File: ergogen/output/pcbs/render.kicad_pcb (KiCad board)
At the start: 2 copper layers, 220.4 x 89.6 mm, 63 parts

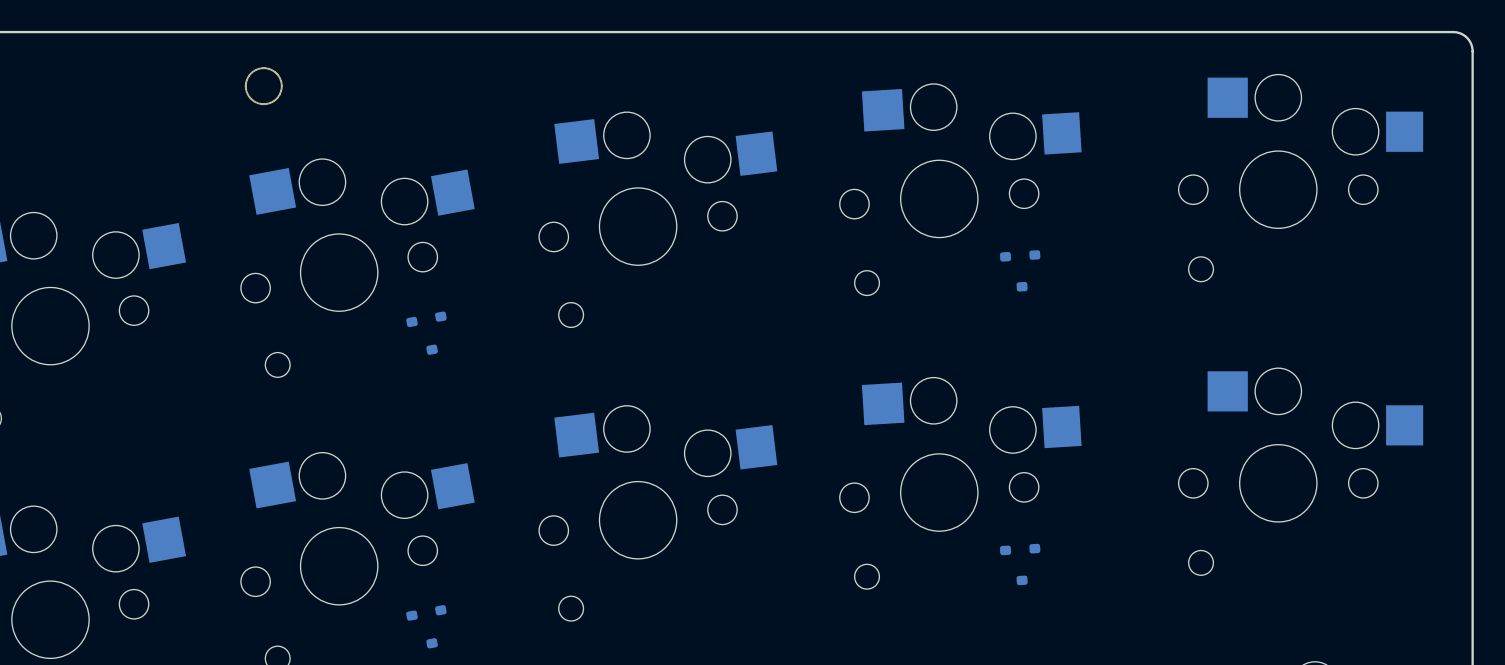
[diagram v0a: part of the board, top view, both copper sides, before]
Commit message: update
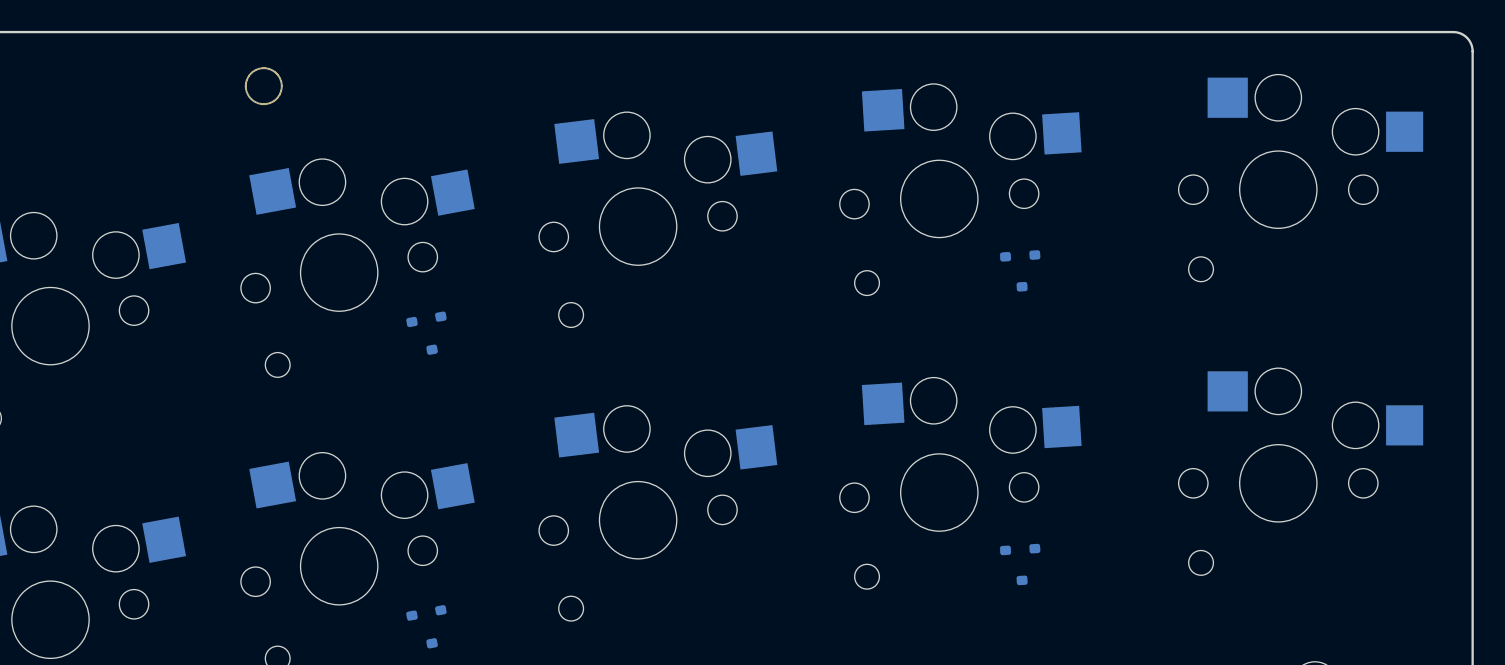
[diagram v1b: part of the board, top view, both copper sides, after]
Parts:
- XX2: footprint 1:conn_molex_pico_front -> conn_molex_pico_front
- moved SW24 141.7 mm to (197.7, 38.0), turned to 0 degrees
- moved SW19 137.6 mm to (-2.38, 38.0), turned to 0 degrees
- moved SW4 116.6 mm to (41.4, 2.39), turned to -7 degrees
- moved SW11 113.5 mm to (21.9, 19.6), turned to -3.5 degrees
- moved SW7 112.7 mm to (173.4, 0.60), turned to 3.5 degrees
- moved SW15 112.7 mm to (173.4, 19.6), turned to 3.5 degrees
- moved SW25 103.9 mm to (178.4, 38.3), turned to 1.75 degrees
- moved SW20 99.5 mm to (16.9, 38.3), turned to -1.75 degrees
- moved SW29 86.7 mm to (55.6, 65.2), turned to -10.5 degrees
- moved SW12 75.5 mm to (41.4, 21.4), turned to -7 degrees
- moved SW16 74.7 mm to (153.9, 21.4), turned to 7 degrees
- moved SW8 74.7 mm to (153.9, 2.39), turned to 7 degrees
- moved SW3 72.8 mm to (21.9, 0.60), turned to -3.5 degrees
- moved SW22 39.4 mm to (56.1, 42.5), turned to -10.5 degrees
- moved SW27 39.4 mm to (139.2, 42.5), turned to 10.5 degrees
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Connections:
- SW10 pad 1: C3 -> C5
- SW10 pad 2: mirror_e_top -> mirror_t_top
- SW11 pad 1: C4 -> C2
- SW11 pad 2: mirror_r_top -> s_home
- SW12 pad 1: C5 -> C3
- SW12 pad 2: mirror_t_top -> d_home
- SW13 pad 1: C2 -> C4
- SW13 pad 2: s_home -> f_home
- SW14 pad 1: C3 -> C5
- SW14 pad 2: d_home -> g_home
- SW15 pad 1: C4 -> C2
- SW15 pad 2: f_home -> mirror_s_home
- SW16 pad 1: C5 -> C3
- SW16 pad 2: g_home -> mirror_d_home
- SW17 pad 1: C2 -> C4
- SW17 pad 2: mirror_s_home -> mirror_f_home
- SW18 pad 1: C3 -> C5
- SW18 pad 2: mirror_d_home -> mirror_g_home
- SW19 pad 1: C4 -> C1
- SW19 pad 2: mirror_f_home -> z_bottom
- SW20 pad 1: C5 -> C2
- SW20 pad 2: mirror_g_home -> x_bottom
- SW21 pad 1: C1 -> C3
- SW21 pad 2: z_bottom -> c_bottom
- SW22 pad 1: C2 -> C4
- SW22 pad 2: x_bottom -> v_bottom
- SW23 pad 1: C3 -> C5
- SW23 pad 2: c_bottom -> b_bottom
- SW24 pad 1: C4 -> C1
- SW24 pad 2: v_bottom -> mirror_z_bottom
- SW25 pad 1: C5 -> C2
- SW25 pad 2: b_bottom -> mirror_x_bottom
- SW26 pad 1: C1 -> C3
- SW26 pad 2: mirror_z_bottom -> mirror_c_bottom
- SW27 pad 1: C2 -> C4
- SW27 pad 2: mirror_x_bottom -> mirror_v_bottom
- SW28 pad 1: C3 -> C5
- SW28 pad 2: mirror_c_bottom -> mirror_b_bottom
- SW29 pad 2: mirror_v_bottom -> base_thumb
- SW3 pad 1: C4 -> C2
- SW3 pad 2: base_thumb -> w_top
- SW30 pad 1: C5 -> C4
- SW30 pad 2: mirror_b_bottom -> mirror_base_thumb
- SW4 pad 1: C4 -> C3
- SW4 pad 2: mirror_base_thumb -> e_top
- SW5 pad 1: C2 -> C4
- SW5 pad 2: w_top -> r_top
- SW6 pad 1: C3 -> C5
- SW6 pad 2: e_top -> t_top
- SW7 pad 1: C4 -> C2
- SW7 pad 2: r_top -> mirror_w_top
- SW8 pad 1: C5 -> C3
- SW8 pad 2: t_top -> mirror_e_top
- SW9 pad 1: C2 -> C4
- SW9 pad 2: mirror_w_top -> mirror_r_top
